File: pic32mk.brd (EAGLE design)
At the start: 110.2 x 85.1 mm, 95 parts, among them IC1 PIC32MK1024MCF100-I_PT, IC10 5.0VDC, IC11 3.3VDC, IC2 ADM3095EBRZ, IC3 TXB0101DCKR, IC4 MAX203ECWP, IC5 TXB0101DCKR, IC6 TXB0101DCKR, IC7 TXB0101DCKR, IC8 TXB0101DCKR, IC9 TXB0101DCKR, J1 1-1586043-4, U1 PMIC-MC33932VW(SOP44), U2 PMIC-MC33932VW(SOP44), U3 ULN2803ADW, U4 REF3425IDBVR, X2 22-23-2081

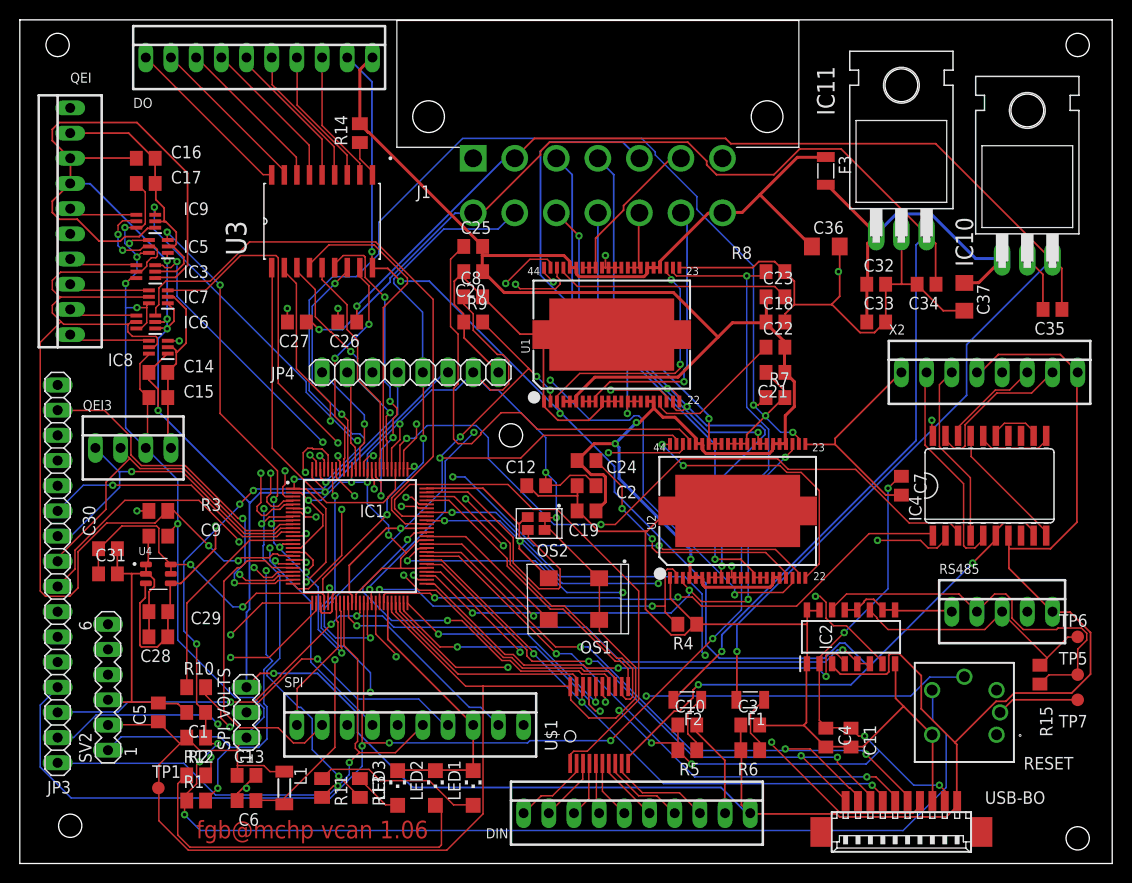
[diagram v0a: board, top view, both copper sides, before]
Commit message: up
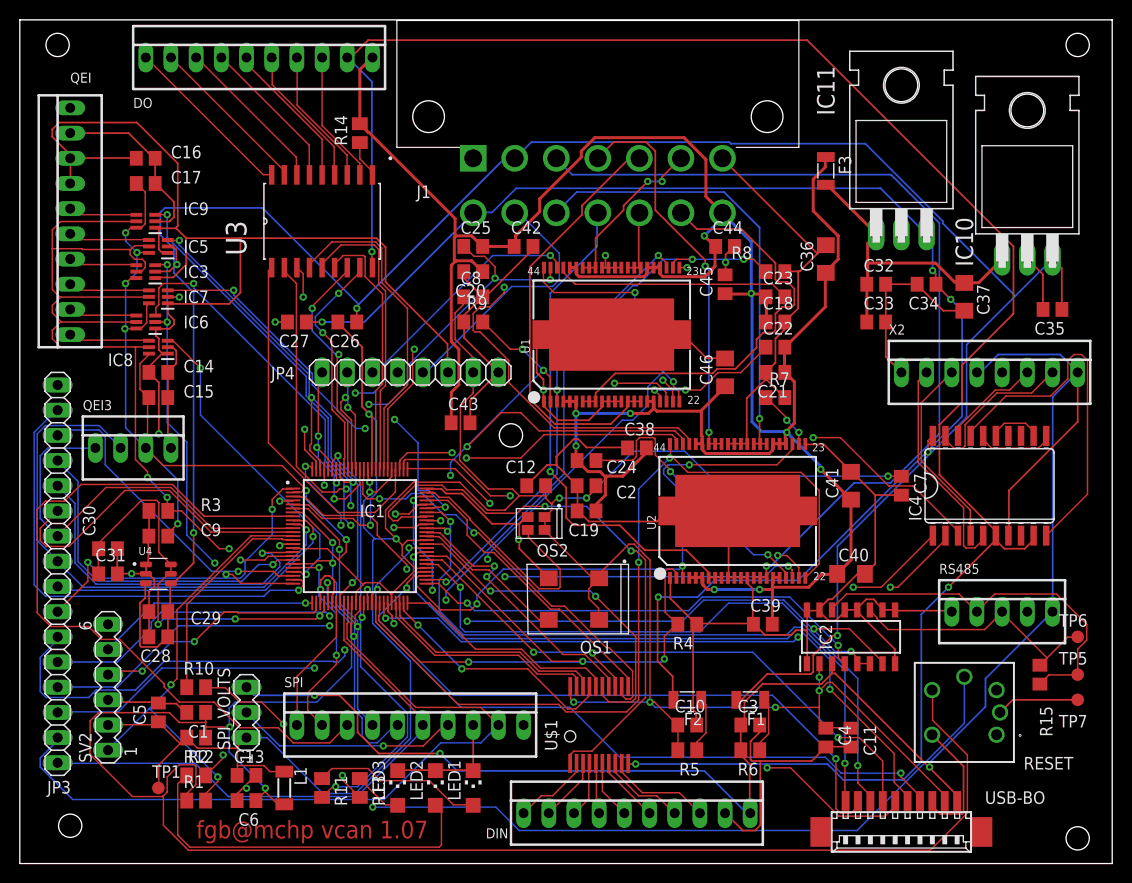
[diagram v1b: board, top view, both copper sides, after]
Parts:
- added C38, C39, C42, C43, C44, C45: 0.1, rcl:C0805
- added C40, C41, C46: 10uf, rcl:C1206
- moved C36 1.27 mm to (77.5, 55.9), turned to 90 degrees
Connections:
- net +24V: now also C38.2, C39.2, C40.1, C41.1, C42.1, C43.1, C44.1, C45.1, C46.1
- net VSS: now also C38.1, C39.1, C40.2, C41.2, C42.2, C43.2, C44.2, C45.2, C46.2
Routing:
- net +24V: track 206.7 -> 266.9 mm, vias 3 -> 9
- net RF13: track 150.1 -> 101.5 mm
- net GND: track 148.6 -> 195.8 mm, vias 4 -> 3
- net RG15: track 147.4 -> 102.5 mm
- net SCK3: track 38.1 -> 76.2 mm, vias 1 -> 0
- net U204: track 53.5 -> 88.2 mm
- net MCLEAR: track 150.4 -> 183.6 mm, vias 6 -> 1
- net +5V: track 198.7 -> 227.2 mm
- net U2RX: track 100.7 -> 75.8 mm
- net RE14: track 73.2 -> 97.0 mm, vias 2 -> 3
- net N$41: track 13.2 -> 36.2 mm
- net VCC: track 341.7 -> 318.9 mm
- net RG6: track 34.6 -> 54.5 mm, vias 0 -> 1
- net PWM4L: track 73.8 -> 56.1 mm
- net RPA14: track 62.1 -> 45.9 mm, vias 0 -> 3
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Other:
- board text added: "fgb@mchp vcan 1.07"
- board text removed: "fgb@mchp vcan 1.06"
